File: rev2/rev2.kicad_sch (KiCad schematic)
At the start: 52 parts, among them J1 Termination, J10 GPIO, J2 CAN1, J3 Termination, J4 CAN2, J5 SWD ASYNC, J6 LIN Pots, J7 AIN, J8 USB_OTG, J9 PWR_USB, SW1 SW_Push, SW2 SW_SPDT, U1 STM32F429ZITx, U2 TJA1051T, U3 TJA1051T, U5 AMS1117-3.3, Y1 16MHz

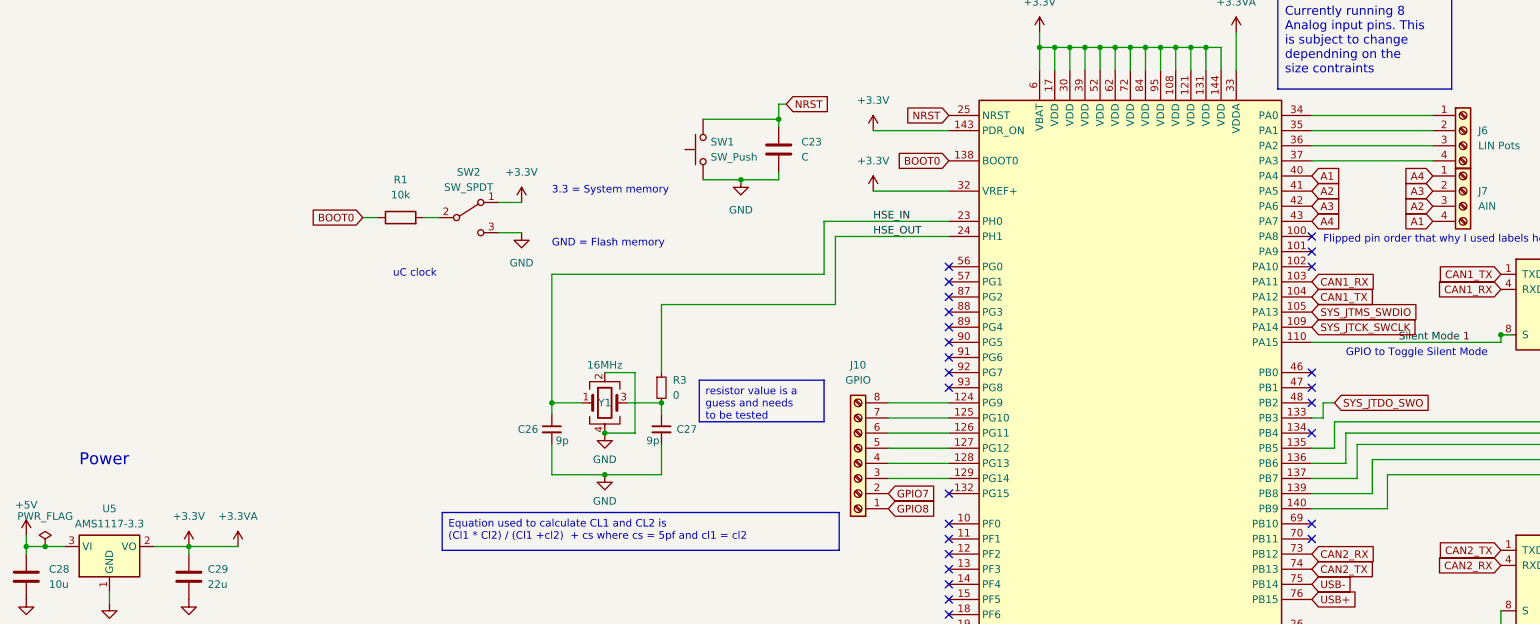
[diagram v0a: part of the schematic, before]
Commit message: added finishing touches to the rev 2 design
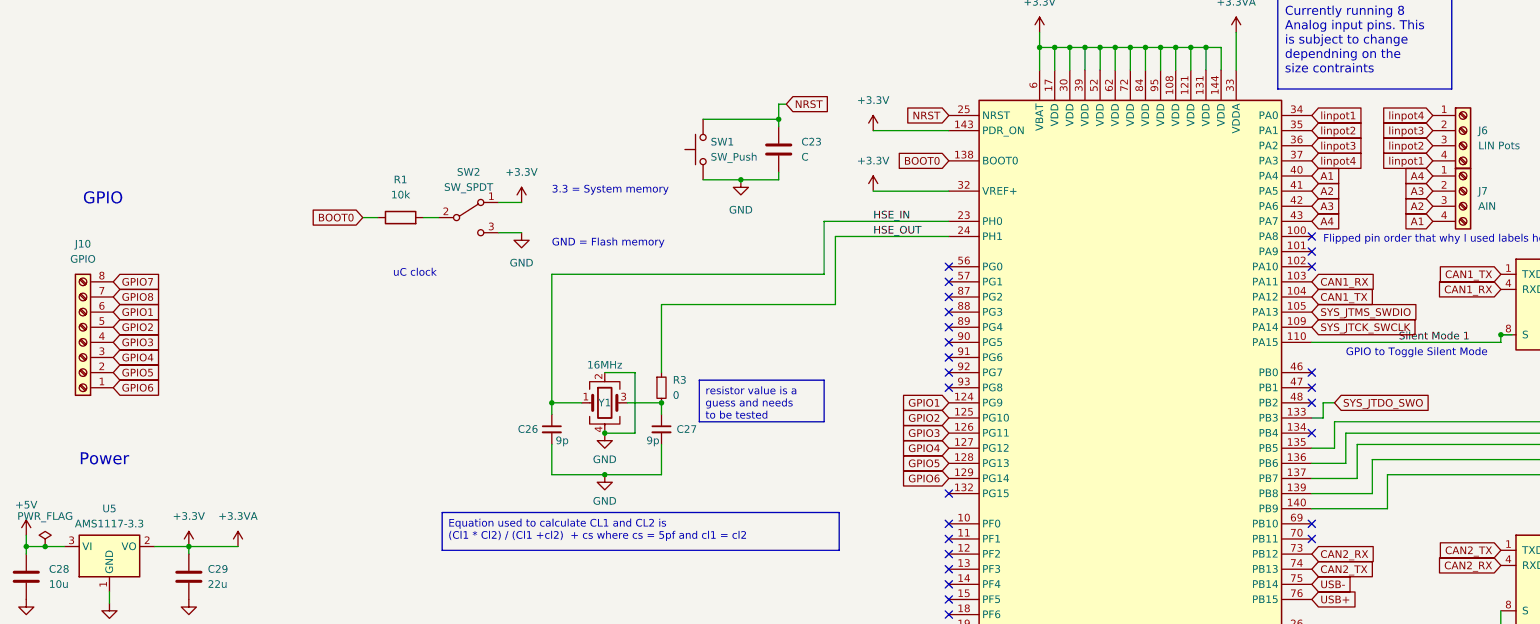
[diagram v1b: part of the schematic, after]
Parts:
- SW2: footprint Button_Switch_SMD:SW_SPDT_CK-JS102011SAQN -> Button_Switch_SMD:SW_SPDT_PCM12
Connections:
- net GPIO7: now also J10.8 (Pin_8); no longer J10.2 (Pin_2)
- net GPIO8: now also J10.7 (Pin_7); no longer J10.1 (Pin_1)
- net GPIO4: now reaches J10.3 (Pin_3)
- net GPIO4: now also U1.127 (PG12); no longer U1.129 (PG14)
- net GPIO3: now reaches J10.4 (Pin_4)
- net GPIO3: now also U1.126 (PG11); no longer U1.128 (PG13)
- net GPIO2: now reaches J10.5 (Pin_5)
- net GPIO2: now also U1.125 (PG10); no longer U1.127 (PG12)
- net GPIO1: now reaches J10.6 (Pin_6)
- net GPIO1: now also U1.124 (PG9); no longer U1.126 (PG11)
- net linpot1: now reaches U1.34 (PA0)
- net linpot1: now also J6.4 (Pin_4); no longer J6.1 (Pin_1)
- net linpot2: now reaches U1.35 (PA1)
- net linpot2: now also J6.3 (Pin_3); no longer J6.2 (Pin_2)
- net linpot3: now reaches U1.36 (PA2)
- net linpot3: now also J6.2 (Pin_2); no longer J6.3 (Pin_3)
- net linpot4: now reaches U1.37 (PA3)
- net linpot4: now also J6.1 (Pin_1); no longer J6.4 (Pin_4)
- new net GPIO5: J10.2 (Pin_2), U1.128 (PG13)
- new net GPIO6: J10.1 (Pin_1), U1.129 (PG14)
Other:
- note added: "GPIO"
- moved on the sheet: J10
